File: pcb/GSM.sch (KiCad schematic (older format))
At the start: 3 parts, among them U12 24V->4V

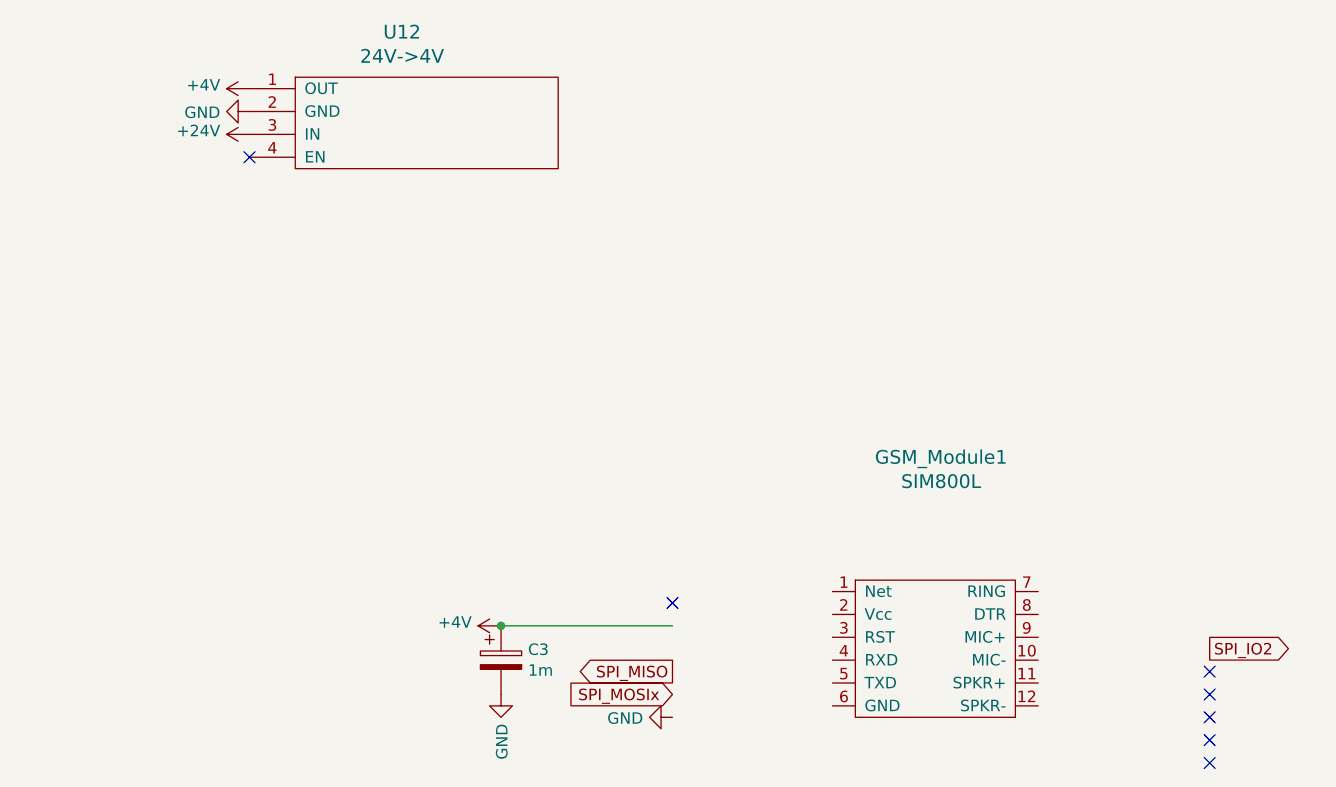
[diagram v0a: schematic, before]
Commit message: Overall unspecific update
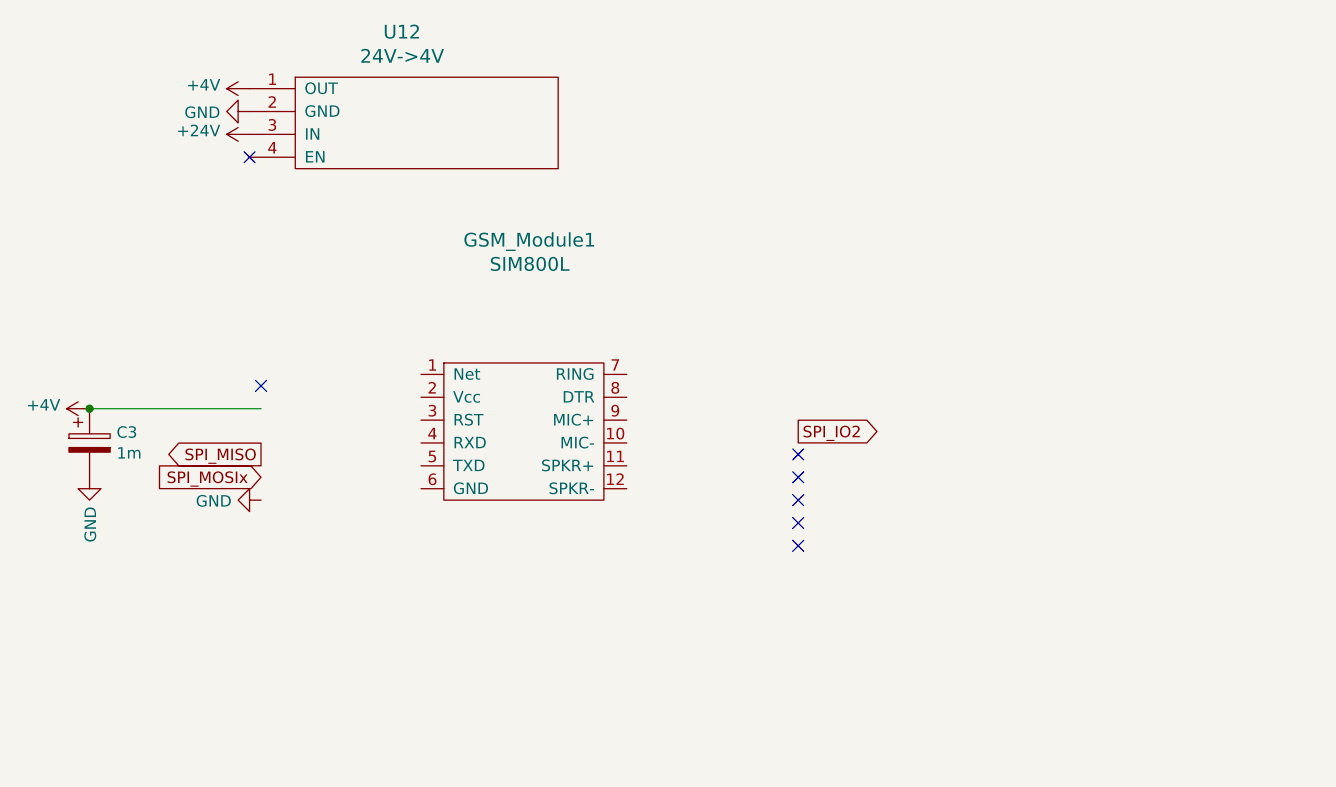
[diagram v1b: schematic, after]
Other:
- moved on the sheet: C3, GSM_Module1
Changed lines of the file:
@@
 L sim800l:SIM800L GSM_Module1
 U 1 1 5F4AA93B
-P 5250 4500
-F 0 "GSM_Module1" H 5275 5387 60  0000 C CNN
-F 1 "SIM800L" H 5275 5281 60  0000 C CNN
-F 2 "smopla:SIM800L" H 5250 4500 60  0001 C CNN
-F 3 "" H 5250 4500 60  0001 C CNN
-	1    5250 4500
+P 3450 3550
+F 0 "GSM_Module1" H 3475 4437 60  0000 C CNN
+F 1 "SIM800L" H 3475 4331 60  0000 C CNN
+F 2 "smopla:SIM800L" H 3450 3550 60  0001 C CNN
+F 3 "" H 3450 3550 60  0001 C CNN
+	1    3450 3550
 	1    0    0    -1
 $EndComp
@@
 L power:GND #PWR0137
 U 1 1 5F4AD790
-P 4100 4750
-F 0 "#PWR0137" H 4100 4500 50  0001 C CNN
-F 1 "GND" V 4105 4622 50  0000 R CNN
-F 2 "" H 4100 4750 50  0001 C CNN
-F 3 "" H 4100 4750 50  0001 C CNN
-	1    4100 4750
+P 2300 3800
+F 0 "#PWR0137" H 2300 3550 50  0001 C CNN
+F 1 "GND" V 2305 3672 50  0000 R CNN
+F 2 "" H 2300 3800 50  0001 C CNN
+F 3 "" H 2300 3800 50  0001 C CNN
+	1    2300 3800
 	0    1    1    0
 $EndComp
-NoConn ~ 6450 4950
-NoConn ~ 6450 4850
-NoConn ~ 6450 4750
-NoConn ~ 6450 4650
-NoConn ~ 6450 4550
-NoConn ~ 4100 4250
-Text GLabel 4100 4550 0    50   Output ~ 0
+NoConn ~ 4650 4000
+NoConn ~ 4650 3900
+NoConn ~ 4650 3800
+NoConn ~ 4650 3700
+NoConn ~ 4650 3600
+NoConn ~ 2300 3300
+Text GLabel 2300 3600 0    50   Output ~ 0
 SPI_MISO
-Text GLabel 6450 4450 2    50   Output ~ 0
+Text GLabel 4650 3500 2    50   Output ~ 0
 SPI_IO2
-Text GLabel 4100 4650 0    50   Input ~ 0
+Text GLabel 2300 3700 0    50   Input ~ 0
 SPI_MOSIx
 $Comp
 L Device:CP C3
 U 1 1 5F507A1A
-P 3350 4500
-F 0 "C3" H 3468 4546 50  0000 L CNN
-F 1 "1m" H 3468 4455 50  0000 L CNN
-F 2 "Capacitor_Tantalum_SMD:CP_EIA-7360-38_Kemet-E_Pad2.25x4.25mm_HandSolder" H 3388 4350 50  0001 C CNN
-F 3 "~" H 3350 4500 50  0001 C CNN
-	1    3350 4500
+P 1550 3550
+F 0 "C3" H 1668 3596 50  0000 L CNN
+F 1 "1m" H 1668 3505 50  0000 L CNN
+F 2 "Capacitor_Tantalum_SMD:CP_EIA-7360-38_Kemet-E_Pad2.25x4.25mm_HandSolder" H 1588 3400 50  0001 C CNN
+F 3 "~" H 1550 3550 50  0001 C CNN
+	1    1550 3550
 	1    0    0    -1
 $EndComp
@@
 L power:+4V #PWR?
 U 1 1 5F508D8F
-P 3350 4350
+P 1550 3400
 AR Path="/5F508D8F" Ref="#PWR?"  Part="1"
 AR Path="/5F49E643/5F508D8F" Ref="#PWR054"  Part="1"
-F 0 "#PWR054" H 3350 4200 50  0001 C CNN
-F 1 "+4V" V 3365 4478 50  0000 L CNN
-F 2 "" H 3350 4350 50  0001 C CNN
-F 3 "" H 3350 4350 50  0001 C CNN
-	1    3350 4350
+F 0 "#PWR054" H 1550 3250 50  0001 C CNN
+F 1 "+4V" V 1565 3528 50  0000 L CNN
+F 2 "" H 1550 3400 50  0001 C CNN
+F 3 "" H 1550 3400 50  0001 C CNN
+	1    1550 3400
 	0    -1   -1   0
 $EndComp
@@
 L power:GND #PWR055
 U 1 1 5F5091E0
-P 3350 4650
-F 0 "#PWR055" H 3350 4400 50  0001 C CNN
-F 1 "GND" V 3355 4522 50  0000 R CNN
-F 2 "" H 3350 4650 50  0001 C CNN
-F 3 "" H 3350 4650 50  0001 C CNN
-	1    3350 4650
+P 1550 3700
+F 0 "#PWR055" H 1550 3450 50  0001 C CNN
+F 1 "GND" V 1555 3572 50  0000 R CNN
+F 2 "" H 1550 3700 50  0001 C CNN
+F 3 "" H 1550 3700 50  0001 C CNN
+	1    1550 3700
 	1    0    0    -1
 $EndComp
 Wire Wire Line
-	4100 4350 3350 4350
-Connection ~ 3350 4350
+	2300 3400 1550 3400
+Connection ~ 1550 3400
 $EndSCHEMATC
